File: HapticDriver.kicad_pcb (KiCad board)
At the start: 4 copper layers, 54.1 x 29 mm, 60 parts, among them J1 Conn_01x02_Pin, J10 Conn_01x02_Pin, J11 Conn_01x02_Pin, J12 Conn_01x02_Pin, J13 Conn_01x02_Pin, J14 USB_C_Receptacle_USB2.0, J2 Conn_01x02_Pin, J3 BATT PWR, J4 Conn_01x02_Pin, J5 Conn_01x02_Pin, J6 Conn_01x02_Pin, J7 Conn_01x02_Pin, J8 Conn_01x02_Pin, J9 Conn_01x02_Pin, SW1 BOOT, SW2 EN, U1 ESP32-S3-WROOM-2, U10 DRV8847SPWR, U11 REG1117-3.3, U2 DRV8847SPWR, U3 74HCT595, U4 74HCT595, U5 74HCT595, U6 DRV8847SPWR, U7 DRV8847SPWR, U8 DRV8847SPWR, U9 DRV8847SPWR

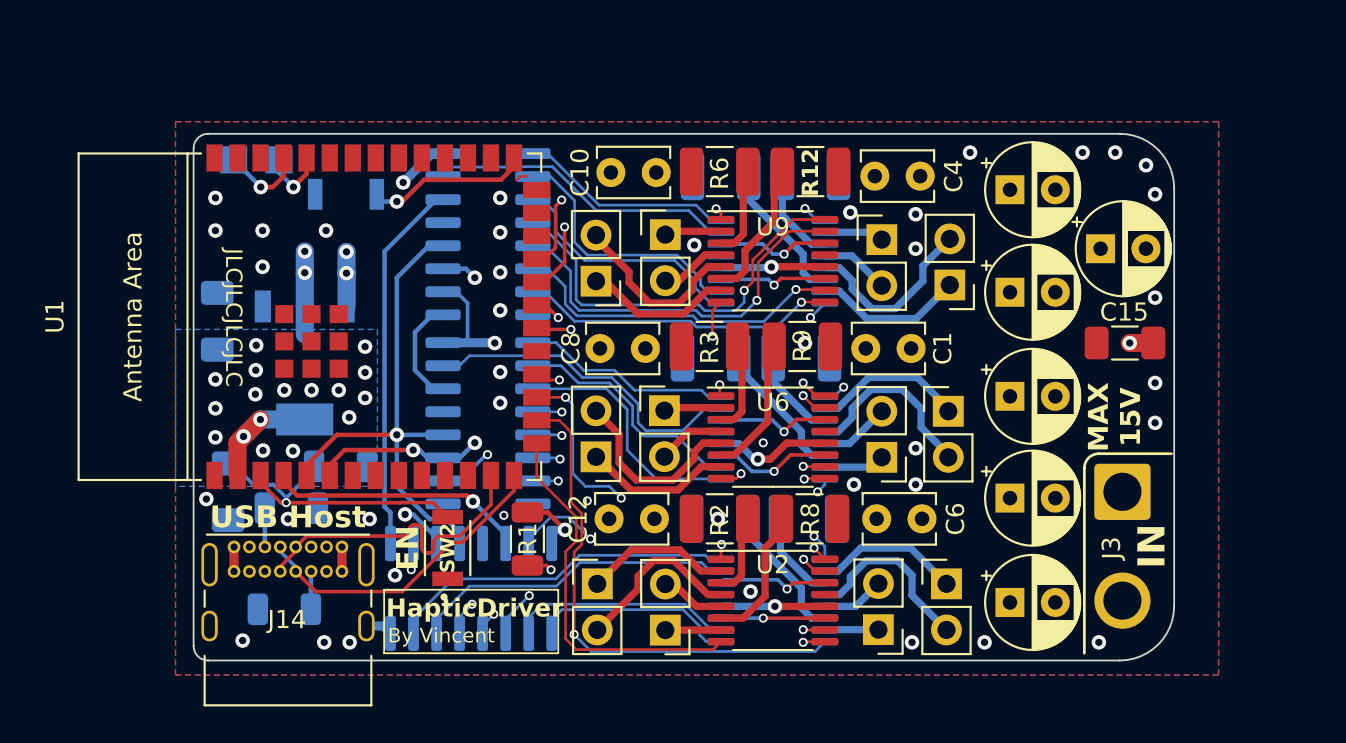
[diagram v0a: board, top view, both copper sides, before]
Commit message: feat: major redesign with better driver and audio, partial routing
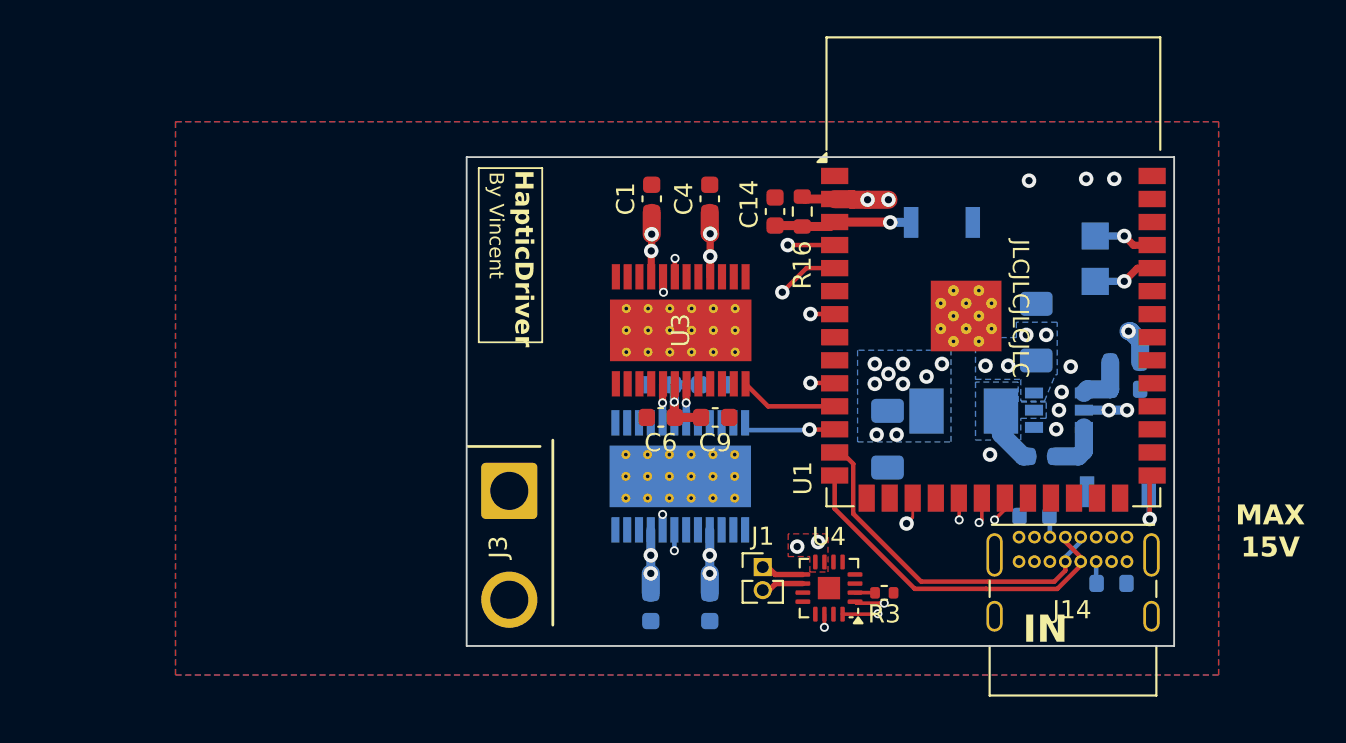
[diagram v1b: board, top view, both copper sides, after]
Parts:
- removed C11: 10uF, Capacitor_THT:CP_Radial_D5.0mm_P2.50mm
- removed C12: 0.1uF, Capacitor_THT:C_Disc_D3.8mm_W2.6mm_P2.50mm
- removed C13, C15: 10uF, Capacitor_SMD:C_1206_3216Metric_Pad1.33x1.80mm_HandSolder
- removed J10, J11, J12, J13, J2, J4, J5, J6, J7, J8, J9: Conn_01x02_Pin, Connector_PinHeader_2.54mm:PinHeader_1x02_P2.54mm_Vertical
- removed R10, R11, R12, R13, R4, R5, R6, R7, R8, R9: 150m, Resistor_SMD:R_1210_3225Metric_Pad1.30x2.65mm_HandSolder
- removed U10, U6, U7, U8, U9: DRV8847SPWR, Package_SO:TSSOP-16_4.4x5mm_P0.65mm
- removed U11: REG1117-3.3, Ti:DCY4
- removed U5: 74HCT595, Package_SO:SOIC-16_3.9x9.9mm_P1.27mm
- added C22: 1uF, Capacitor_SMD:C_0603_1608Metric, B.Cu at (136.4, 97.8)
- added L1: 3.3uH, Changjiang:L_Changjiang_FXL0530-3R3-M, B.Cu at (150.4, 87.0)
- added U12: DRV8912QPWPRQ1, Ti:PWP0024N_N, B.Cu at (134.8, 90.5)
- C1, C6: footprint Capacitor_THT:C_Disc_D3.8mm_W2.6mm_P2.50mm -> Capacitor_SMD:C_0603_1608Metric
- C10: value 0.1uF -> 100nF; footprint Capacitor_THT:C_Disc_D3.8mm_W2.6mm_P2.50mm -> Capacitor_SMD:C_0603_1608Metric; moved to B.Cu
- C14: footprint Capacitor_SMD:C_1206_3216Metric_Pad1.33x1.80mm_HandSolder -> Capacitor_SMD:C_0603_1608Metric; moved to F.Cu
- C2, C3, C5: value 10uF -> 0.1uF; footprint Capacitor_THT:CP_Radial_D5.0mm_P2.50mm -> Capacitor_SMD:C_0603_1608Metric; moved to B.Cu
- C4: value 0.1uF -> 1uF; footprint Capacitor_THT:C_Disc_D3.8mm_W2.6mm_P2.50mm -> Capacitor_SMD:C_0603_1608Metric
- C7: footprint Capacitor_THT:CP_Radial_D5.0mm_P2.50mm -> Capacitor_SMD:C_1206_3216Metric_Pad1.33x1.80mm_HandSolder; moved to B.Cu
- C8: value 0.1uF -> 10uF; footprint Capacitor_THT:C_Disc_D3.8mm_W2.6mm_P2.50mm -> Capacitor_SMD:C_1206_3216Metric_Pad1.33x1.80mm_HandSolder; moved to B.Cu
- C9: value 10uF -> 0.1uF; footprint Capacitor_THT:CP_Radial_D5.0mm_P2.50mm -> Capacitor_SMD:C_0603_1608Metric
- J1: value Conn_01x02_Pin -> Conn_01x02_Socket; footprint Connector_PinHeader_2.54mm:PinHeader_1x02_P2.54mm_Vertical -> Connector_PinHeader_1.27mm:PinHeader_1x02_P1.27mm_Vertical
- R1: value 5K1 -> R; footprint Resistor_SMD:R_1206_3216Metric -> Resistor_SMD:R_0603_1608Metric; moved to B.Cu
- R14, R15: footprint Resistor_SMD:R_1206_3216Metric -> Resistor_SMD:R_0603_1608Metric
- R16: footprint Resistor_SMD:R_1206_3216Metric -> Resistor_SMD:R_0603_1608Metric; moved to F.Cu
- R2: value 150m -> R; footprint Resistor_SMD:R_1210_3225Metric_Pad1.30x2.65mm_HandSolder -> Resistor_SMD:R_0603_1608Metric; moved to B.Cu
- R3: value 150m -> R; footprint Resistor_SMD:R_1210_3225Metric_Pad1.30x2.65mm_HandSolder -> Resistor_SMD:R_0402_1005Metric
- SW2: moved to B.Cu
- U1: footprint PCM_Espressif:ESP32-S3-WROOM-2 -> RF_Module:ESP32-S3-WROOM-1
- U2: value DRV8847SPWR -> TPS561201DDCR; footprint Package_SO:TSSOP-16_4.4x5mm_P0.65mm -> Ti:DDC0006A_N; moved to B.Cu
- U3: value 74HCT595 -> DRV8912QPWPRQ1; footprint Package_SO:SOIC-16_3.9x9.9mm_P1.27mm -> Ti:PWP0024N_N; moved to F.Cu
- U4: value 74HCT595 -> MAX98357A; footprint Package_SO:SOIC-16_3.9x9.9mm_P1.27mm -> Package_DFN_QFN:TQFN-16-1EP_3x3mm_P0.5mm_EP1.23x1.23mm; moved to F.Cu
- moved TP1 47.7 mm to (157.7, 77.3), turned to 90 degrees
- moved R15 45.6 mm to (158.6, 96.5), turned to 180 degrees
- moved SW1 45.6 mm to (158.9, 91.4)
- moved TP2 45.5 mm to (157.7, 79.8), turned to 90 degrees
- moved J14 43.3 mm to (153.5, 93.9)
- moved R14 41.0 mm to (154.3, 92.8), turned to 0 degrees
- moved U1 34.8 mm to (152.1, 79.2), turned to 0 degrees
- moved R1 34.4 mm to (159.3, 84.2), turned to 180 degrees
- moved C14 33.9 mm to (140.1, 76.0), turned to 90 degrees
- moved J3 33.8 mm to (125.4, 91.3)
- moved SW2 32.6 mm to (149.2, 76.5), turned to 180 degrees
- moved C3 31.7 mm to (133.2, 97.8), turned to -90 degrees
- moved R16 29.1 mm to (141.6, 76.0), turned to -90 degrees
- moved U4 27.1 mm to (143.0, 96.7)
- moved C10 26.4 mm to (154.8, 89.5)
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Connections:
- C10 pad 1: +BATT -> Net-(U2-VBST)
- C10 pad 2: GND -> Net-(U2-SW)
- C2 pad 1: +BATT -> +3V3
- C5 pad 1: +BATT -> +3V3
- C6 pad 1: +BATT -> +3V3
- C8 pad 1: +BATT -> +3V3
- C9 pad 1: +BATT -> +3V3
- R1 pad 1: /DRV_SDA -> +3V3
- R1 pad 2: +3V3 -> Net-(U2-VFB)
- R2 pad 1: Net-(U2-ISEN12) -> Net-(U2-VFB)
- R3 pad 1: Net-(U6-ISEN12) -> GND
- R3 pad 2: GND -> Net-(U4-GAIN_SLOT)
- U1 pad 10: unconnected-(U1-GPIO17/U1TXD/ADC2_CH6-Pad10) -> /DRV_MISO
- U1 pad 11: unconnected-(U1-GPIO18/U1RXD/ADC2_CH7/CLK_OUT3-Pad11) -> /nFAULT_2
- U1 pad 12: unconnected-(U1-GPIO8/TOUCH8/ADC1_CH7/SUBSPICS1-Pad12) -> /nFAULT_1
- U1 pad 15: /nFAULT_1 -> unconnected-(U1-GPIO3/TOUCH3/ADC1_CH2-Pad15)
- U1 pad 16: /nFAULT_6 -> unconnected-(U1-GPIO46-Pad16)
- U1 pad 17: /nFAULT_4 -> /DRV_CS_1
- U1 pad 18: /nFAULT_2 -> unconnected-(U1-GPIO10/TOUCH10/ADC1_CH9/FSPICS0/FSPIIO4/SUBSPICS0-Pad18)
- U1 pad 19: unconnected-(U1-GPIO11/TOUCH11/ADC2_CH0/FSPID/FSPIIO5/SUBSPID-Pad19) -> /I2S_DIN
- U1 pad 20: /nFAULT_3 -> /I2S_BCLK
- U1 pad 21: /nFAULT_5 -> /I2S_WCLK
- U1 pad 4: /I2S_DATA -> /DRV_SCK
- U1 pad 5: /I2S_WS -> /DRV_CS_2
- U1 pad 6: /I2S_BCLK -> unconnected-(U1-GPIO6/TOUCH6/ADC1_CH5-Pad6)
- U1 pad 7: unconnected-(U1-GPIO7/TOUCH7/ADC1_CH6-Pad7) -> /DRV_MOSI
- U2 pad 1: +3V3 -> GND
- U2 pad 2: Net-(J1-Pin_1) -> Net-(U2-SW)
- U2 pad 3: Net-(U2-ISEN12) -> +BATT
- U2 pad 4: Net-(J1-Pin_2) -> Net-(U2-VFB)
- U2 pad 5: Net-(J2-Pin_2) -> +BATT
- U2 pad 6: Net-(U2-ISEN34) -> Net-(U2-VBST)
- U3 pad 1: /D6_IN3 -> GND
- U3 pad 10: +3V3 -> unconnected-(U3-OUT6-Pad10)
- U3 pad 11: /I2S_BCLK -> unconnected-(U3-OUT4-Pad11)
- U3 pad 12: /I2S_WS -> /nFAULT_2
- U3 pad 14: /I2S_DATA -> unconnected-(U3-OUT3-Pad14)
- U3 pad 15: /D1_IN1 -> unconnected-(U3-OUT10-Pad15)
- U3 pad 16: +3V3 -> +BATT
- U3 pad 2: /D6_IN4 -> unconnected-(U3-OUT1-Pad2)
- U3 pad 3: /D1_IN2 -> unconnected-(U3-OUT5-Pad3)
- U3 pad 4: /D1_IN3 -> unconnected-(U3-OUT7-Pad4)
- U3 pad 5: /D1_IN4 -> /DRV_MOSI
- U3 pad 6: /D6_IN2 -> +3V3
- U3 pad 7: /D6_IN1 -> /DRV_MISO
- U3 pad 8: GND -> /Driver 2/nSLEEP
- U3 pad 9: Net-(U3-QH') -> unconnected-(U3-OUT9-Pad9)
- U4 pad 1: /D3_IN1 -> /I2S_DIN
- U4 pad 10: +3V3 -> Net-(J1-Pin_2)
- U4 pad 11: /I2S_BCLK -> GND
- U4 pad 12: /I2S_WS -> unconnected-(U4-NC-Pad12)
- U4 pad 13: GND -> unconnected-(U4-NC-Pad13)
- U4 pad 14: Net-(U3-QH') -> /I2S_WCLK
- U4 pad 15: /D3_IN2 -> GND
- U4 pad 16: +3V3 -> /I2S_BCLK
- U4 pad 2: /D3_IN4 -> Net-(U4-GAIN_SLOT)
- U4 pad 3: /D3_IN3 -> GND
- U4 pad 4: /D5_IN1 -> unconnected-(U4-~{SD_MODE}-Pad4)
- U4 pad 5: /D5_IN2 -> unconnected-(U4-NC-Pad5)
- U4 pad 6: /D5_IN4 -> unconnected-(U4-NC-Pad6)
- U4 pad 7: /D5_IN3 -> +3V3
- U4 pad 8: GND -> +3V3
- U4 pad 9: Net-(U4-QH') -> Net-(J1-Pin_1)
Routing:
- net /DRV_SDA: track 72.0 -> 0.00 mm, vias 5 -> 0
- net +3V3: track 79.7 -> 13.8 mm, vias 30 -> 15
- net /DRV_SCL: track 54.9 -> 0.00 mm, vias 4 -> 0
- net /nFAULT_6: track 28.2 -> 0.00 mm, vias 1 -> 0
- net /I2S_WS: track 28.1 -> 0.00 mm, vias 1 -> 0
- net /DRV_SCK: track 0.00 -> 26.1 mm, vias 0 -> 3
- net /D5_IN1: track 22.6 -> 0.00 mm, vias 1 -> 0
- net /D5_IN2: track 21.8 -> 0.00 mm, vias 1 -> 0
- net /D1_IN4: track 21.3 -> 0.00 mm, vias 2 -> 0
- net /nFAULT_4: track 21.0 -> 0.00 mm, vias 3 -> 0
- net Net-(U3-QH'): track 20.6 -> 0.00 mm
- net /D1_IN3: track 20.4 -> 0.00 mm, vias 2 -> 0
- net /D1_IN2: track 20.0 -> 0.00 mm, vias 2 -> 0
- net /D6_IN1: track 19.3 -> 0.00 mm
- net /D5_IN4: track 18.6 -> 0.00 mm, vias 1 -> 0
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- added copper zone on F.Cu, net +3V3
- added copper zone on B.Cu, net +BATT
- added copper zone on B.Cu, net Net-(U2-SW)
- removed copper zone on In1.Cu, net GND
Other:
- board size 54.1 x 29 mm -> 39 x 27 mm
- board text removed: "USB Host"
